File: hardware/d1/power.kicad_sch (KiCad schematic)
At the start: 44 parts, among them U10 BLM15PX601SN1D, U11 TPS7A2033PDBVR, U12 TPS7A2018PDBVR, U13 TPS7A2018PDBVR, U7 TPS7A2018PDBVR, U8 TPS7A2033PDBVR, U9 TPS560430XFDBVR

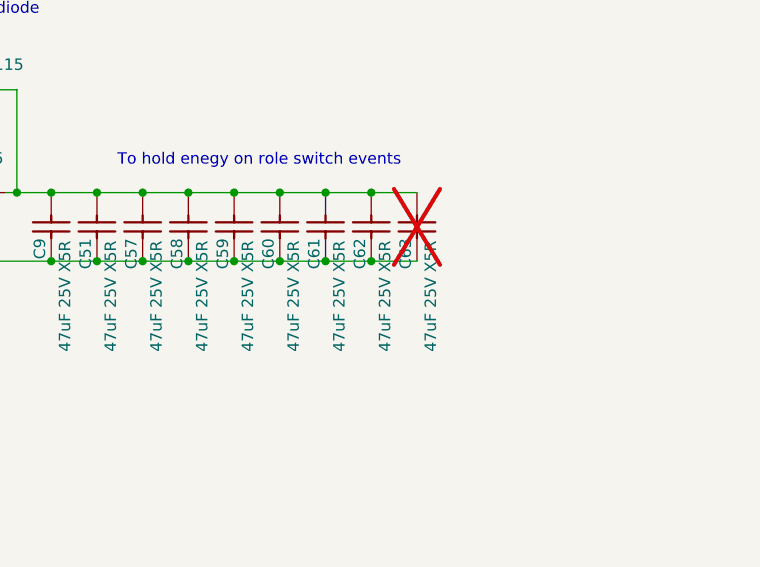
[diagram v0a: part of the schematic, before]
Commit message: Almost done tracing
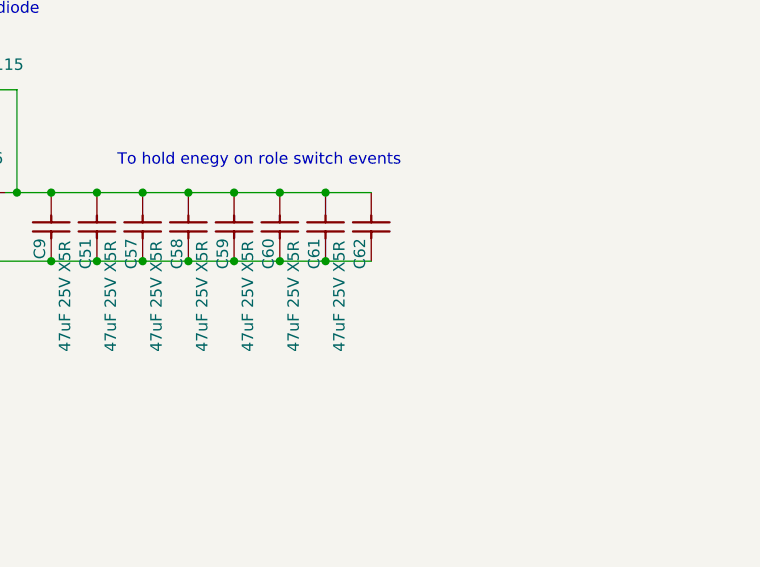
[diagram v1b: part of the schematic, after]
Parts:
- removed C63: 47uF 25V X5R, Capacitor_SMD:C_1206_3216Metric, symbol JLCImport:C3216X5R1E476MTJ00E
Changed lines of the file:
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@@
 	)
 	(junction
-		(at 167.64 36.83)
-		(diameter 0)
-		(color 0 0 0 0)
-	)
-	(junction
 		(at 166.37 107.95)
 		(diameter 0)
@@
 	)
 	(junction
-		(at 167.64 44.45)
-		(diameter 0)
-		(color 0 0 0 0)
-	)
-	(junction
 		(at 191.77 92.71)
 		(diameter 0)
@@
 	(wire
 		(pts
-			(xy 167.64 44.45) (xy 172.72 44.45)
-		)
-		(stroke
-			(width 0)
-			(type default)
-		)
-	)
-	(wire
-		(pts
 			(xy 81.28 50.8) (xy 87.63 50.8)
 		)
@@
 	(wire
 		(pts
-			(xy 167.64 36.83) (xy 172.72 36.83)
-		)
-		(stroke
-			(width 0)
-			(type default)
-		)
-	)
-	(wire
-		(pts
 			(xy 134.62 106.68) (xy 134.62 111.76)
 		)
@@
 		(property "Value" "47uF 25V X5R"
 			(at 169.164 42.164 0)
+			(hide yes)
 			(show_name no)
 			(do_not_autoplace no)
@@
 					(unit 1)
 				)
-			)
-		)
-	)
-	(symbol
-		(lib_id "JLCImport:C3216X5R1E476MTJ00E")
-		(at 172.72 40.64 90)
-		(unit 1)
-		(body_style 1)
-		(exclude_from_sim no)
-		(in_bom yes)
-		(on_board yes)
-		(in_pos_files yes)
-		(dnp yes)
-		(property "Reference" "C63"
-			(at 171.45 41.91 0)
-			(show_name no)
-			(do_not_autoplace no)
-			(effects
-				(font
-					(size 1.27 1.27)
-				)
-				(justify right)
-			)
-		)
-		(property "Value" "47uF 25V X5R"
-			(at 174.244 42.164 0)
-			(show_name no)
-			(do_not_autoplace no)
-			(effects
-				(font
-					(size 1.27 1.27)
-				)
-				(justify right)
-			)
-		)
-		(property "Footprint" "Capacitor_SMD:C_1206_3216Metric"
-			(at 172.72 40.64 0)
-			(hide yes)
-			(show_name no)
-			(do_not_autoplace no)
-			(effects
-				(font
-					(size 1.27 1.27)
-				)
-			)
-		)
-		(property "Datasheet" "https://www.lcsc.com/datasheet/lcsc_datasheet_2304140030_TDK-C3216X5R1E476MTJ00E_C76659.pdf"
-			(at 172.72 40.64 0)
-			(hide yes)
-			(show_name no)
-			(do_not_autoplace no)
-			(effects
-				(font
-					(size 1.27 1.27)
-				)
-			)
-		)
-		(property "Description" "25V 47uF X5R ±20% 1206 Multilayer Ceramic Capacitors MLCC - SMD/SMT ROHS"
-			(at 172.72 40.64 0)
-			(hide yes)
-			(show_name no)
-			(do_not_autoplace no)
-			(effects
-				(font
-					(size 1.27 1.27)
-				)
-			)
-		)
-		(property "LCSC" "C76659"
-			(at 172.72 40.64 0)
-			(hide yes)
-			(show_name no)
-			(do_not_autoplace no)
-			(effects
-				(font
-					(size 1.27 1.27)
-				)
-			)
-		)
-		(property "Manufacturer" "TDK"
-			(at 172.72 40.64 0)
-			(hide yes)
-			(show_name no)
-			(do_not_autoplace no)
-			(effects
-				(font
-					(size 1.27 1.27)
-				)
-			)
-		)
-		(property "Manufacturer Part" "C3216X5R1E476MTJ00E"
-			(at 172.72 40.64 0)
-			(hide yes)
-			(show_name no)
-			(do_not_autoplace no)
-			(effects
-				(font
-					(size 1.27 1.27)
-				)
-			)
-		)
-		(pin "1"
-		)
-		(pin "2"
-		)
-		(instances
-			(project "DrunkEarPhoneAdapter"
-				(path "/df940915-8af0-46f9-b18a-23d4684ae671/bea21a31-aee1-46f9-b13e-ece764487360"
-					(reference "C63")
-					(unit 1)
-				)
